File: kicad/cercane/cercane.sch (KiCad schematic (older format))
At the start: 2 parts, among them U1 ATtiny45-20SU, U2 NRF24L01_Breakout

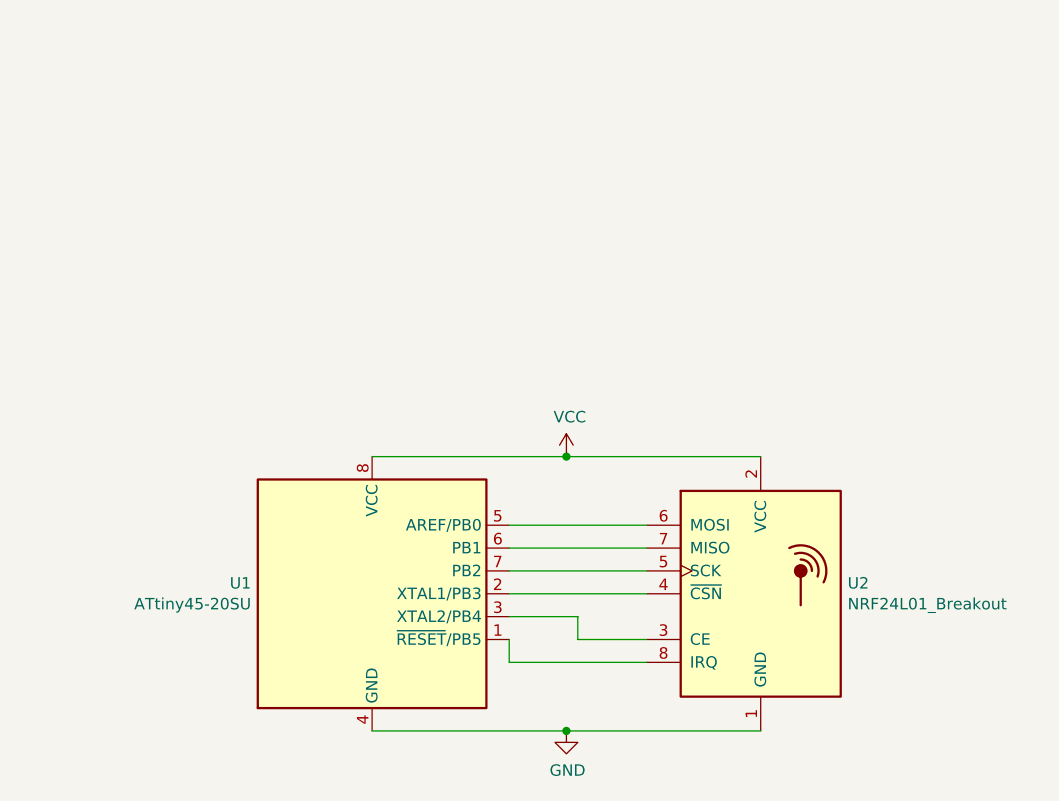
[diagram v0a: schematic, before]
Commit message: new PCB
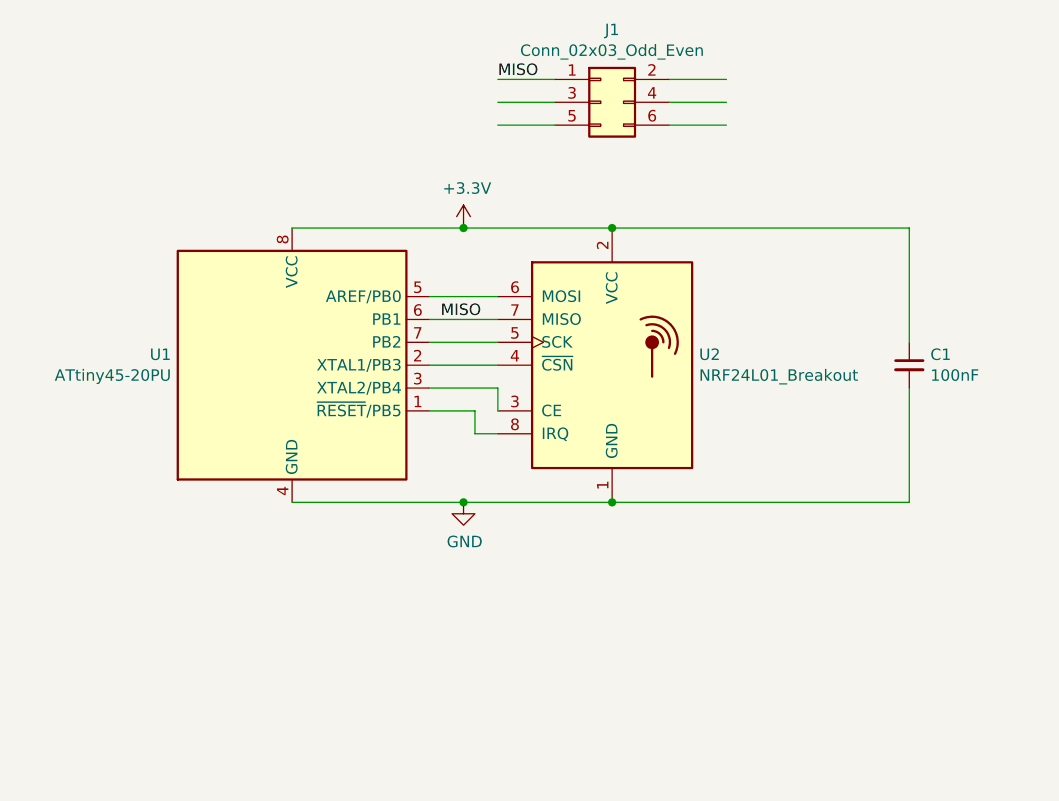
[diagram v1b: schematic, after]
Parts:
- removed U1: ATtiny45-20SU, ATTINY85-20SU:SOIC127P798X216-8N, symbol MCU_Microchip_ATtiny:ATtiny45-20SU
- added C1: 100nF, Capacitor_SMD:C_1206_3216Metric, symbol Device:C_Small
- added J1: Conn_02x03_Odd_Even, Connector_PinSocket_2.54mm:PinSocket_2x03_P2.54mm_Vertical_SMD, symbol Connector_Generic:Conn_02x03_Odd_Even
- added U1: ATtiny45-20PU, ATTINY45-20PU:DIP787W46P254L927H533Q8, symbol MCU_Microchip_ATtiny:ATtiny45-20PU
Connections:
- net labels added: +3.3V, MISO
- net labels removed: VCC
- wire segments 13 -> 23
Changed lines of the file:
@@
 Comment4 ""
 $EndDescr
-Wire Wire Line
-	5600 3400 6200 3400
-Wire Wire Line
-	5600 3300 6200 3300
-Wire Wire Line
-	5600 3200 6200 3200
 $Comp
-L RF:NRF24L01_Breakout U2
-U 1 1 60DE15C7
-P 6700 3500
-F 0 "U2" H 7080 3546 50  0000 L CNN
-F 1 "NRF24L01_Breakout" H 7080 3455 50  0000 L CNN
-F 2 "RF_Module:nRF24L01_Breakout" H 6850 4100 50  0001 L CIN
-F 3 "http://www.nordicsemi.com/eng/content/download/2730/34105/file/nRF24L01_Product_Specification_v2_0.pdf" H 6700 3400 50  0001 C CNN
-	1    6700 3500
+L MCU_Microchip_ATtiny:ATtiny45-20PU U1
+U 1 1 60DE1A7E
+P 4650 2500
+F 0 "U1" H 4121 2546 50  0000 R CNN
+F 1 "ATtiny45-20PU" H 4121 2455 50  0000 R CNN
+F 2 "ATTINY45-20PU:DIP787W46P254L927H533Q8" H 4650 2500 50  0001 C CIN
+F 3 "http://ww1.microchip.com/downloads/en/DeviceDoc/atmel-2586-avr-8-bit-microcontroller-attiny25-attiny45-attiny85_datasheet.pdf" H 4650 2500 50  0001 C CNN
+	1    4650 2500
 	1    0    0    -1
 $EndComp
 $Comp
-L MCU_Microchip_ATtiny:ATtiny45-20SU U1
-U 1 1 60DE0B3D
-P 5000 3500
-F 0 "U1" H 4471 3546 50  0000 R CNN
-F 1 "ATtiny45-20SU" H 4471 3455 50  0000 R CNN
-F 2 "ATTINY85-20SU:SOIC127P798X216-8N" H 5000 3500 50  0001 C CIN
-F 3 "http://ww1.microchip.com/downloads/en/DeviceDoc/atmel-2586-avr-8-bit-microcontroller-attiny25-attiny45-attiny85_datasheet.pdf" H 5000 3500 50  0001 C CNN
-	1    5000 3500
+L RF:NRF24L01_Breakout U2
+U 1 1 60DE2CD2
+P 6050 2500
+F 0 "U2" H 6430 2546 50  0000 L CNN
+F 1 "NRF24L01_Breakout" H 6430 2455 50  0000 L CNN
+F 2 "RF_Module:nRF24L01_Breakout" H 6200 3100 50  0001 L CIN
+F 3 "http://www.nordicsemi.com/eng/content/download/2730/34105/file/nRF24L01_Product_Specification_v2_0.pdf" H 6050 2400 50  0001 C CNN
+	1    6050 2500
 	1    0    0    -1
 $EndComp
 Wire Wire Line
-	5600 3500 6200 3500
+	5550 2200 5250 2200
 Wire Wire Line
-	5600 3600 5900 3600
+	5550 2300 5250 2300
 Wire Wire Line
-	5900 3600 5900 3700
+	5550 2400 5250 2400
 Wire Wire Line
-	5900 3700 6200 3700
+	5550 2500 5250 2500
 Wire Wire Line
-	5600 3700 5600 3800
+	5250 2600 5550 2600
 Wire Wire Line
-	5600 3800 6200 3800
+	5550 2600 5550 2700
+Wire Wire Line
+	5250 2700 5450 2700
+Wire Wire Line
+	5450 2700 5450 2800
+Wire Wire Line
+	5450 2800 5550 2800
+Wire Wire Line
+	4650 3100 5400 3100
 $Comp
-L power:VCC #PWR0101
-U 1 1 60E0A716
-P 5850 2900
-F 0 "#PWR0101" H 5850 2750 50  0001 C CNN
-F 1 "VCC" H 5865 3073 50  0000 C CNN
-F 2 "" H 5850 2900 50  0001 C CNN
-F 3 "" H 5850 2900 50  0001 C CNN
-	1    5850 2900
+L power:GND #PWR0101
+U 1 1 60DE48AA
+P 5400 3100
+F 0 "#PWR0101" H 5400 2850 50  0001 C CNN
+F 1 "GND" H 5405 2927 50  0000 C CNN
+F 2 "" H 5400 3100 50  0001 C CNN
+F 3 "" H 5400 3100 50  0001 C CNN
+	1    5400 3100
 	1    0    0    -1
 $EndComp
+Connection ~ 5400 3100
+Wire Wire Line
+	5400 3100 6050 3100
 $Comp
-L power:GND #PWR0102
-U 1 1 60E0AE4F
-P 5850 4100
-F 0 "#PWR0102" H 5850 3850 50  0001 C CNN
-F 1 "GND" H 5855 3927 50  0000 C CNN
-F 2 "" H 5850 4100 50  0001 C CNN
-F 3 "" H 5850 4100 50  0001 C CNN
-	1    5850 4100
+L power:+3.3V #PWR0102
+U 1 1 60DE4DCC
+P 5400 1900
+F 0 "#PWR0102" H 5400 1750 50  0001 C CNN
+F 1 "+3.3V" H 5415 2073 50  0000 C CNN
+F 2 "" H 5400 1900 50  0001 C CNN
+F 3 "" H 5400 1900 50  0001 C CNN
+	1    5400 1900
 	1    0    0    -1
 $EndComp
 Wire Wire Line
-	5000 2900 5850 2900
+	4650 1900 5400 1900
 Wire Wire Line
-	6700 2900 5850 2900
-Connection ~ 5850 2900
+	6050 1900 5400 1900
+Connection ~ 5400 1900
+$Comp
+L Device:C_Small C1
+U 1 1 60E49E1A
+P 7350 2500
+F 0 "C1" H 7442 2546 50  0000 L CNN
+F 1 "100nF" H 7442 2455 50  0000 L CNN
+F 2 "Capacitor_SMD:C_1206_3216Metric" H 7350 2500 50  0001 C CNN
+F 3 "~" H 7350 2500 50  0001 C CNN
+	1    7350 2500
+	1    0    0    -1
+$EndComp
 Wire Wire Line
-	5000 4100 5850 4100
+	6050 1900 7350 1900
 Wire Wire Line
-	6700 4100 5850 4100
-Connection ~ 5850 4100
+	7350 1900 7350 2400
+Connection ~ 6050 1900
+Wire Wire Line
+	7350 2600 7350 3100
+Wire Wire Line
+	7350 3100 6050 3100
+Connection ~ 6050 3100
+$Comp
+L Connector_Generic:Conn_02x03_Odd_Even J1
+U 1 1 60E4B806
+P 6000 1350
+F 0 "J1" H 6050 1667 50  0000 C CNN
+F 1 "Conn_02x03_Odd_Even" H 6050 1576 50  0000 C CNN
+F 2 "Connector_PinSocket_2.54mm:PinSocket_2x03_P2.54mm_Vertical_SMD" H 6000 1350 50  0001 C CNN
+F 3 "~" H 6000 1350 50  0001 C CNN
+	1    6000 1350
+	1    0    0    -1
+$EndComp
+Wire Wire Line
+	5800 1250 5550 1250
+Wire Wire Line
+	5800 1350 5550 1350
+Wire Wire Line
+	5800 1450 5550 1450
+Wire Wire Line
+	6300 1250 6550 1250
+Wire Wire Line
+	6300 1350 6550 1350
+Wire Wire Line
+	6300 1450 6550 1450
+Text Label 5550 1250 0    50   ~ 0
+MISO
+Text Label 5300 2300 0    50   ~ 0
+MISO
 $EndSCHEMATC
